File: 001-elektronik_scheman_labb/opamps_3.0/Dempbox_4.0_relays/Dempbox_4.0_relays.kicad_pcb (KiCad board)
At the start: 2 copper layers, 86 x 54.5 mm, 41 parts, among them J1 Test_probe, J10 Mätinstrument, J11 J_SW_SIGNAL, J2 TO_Focusrite_input, J3 OP_AMP_PWR, J4 Speaker, J9 Mätinstrument, U2 OPA134

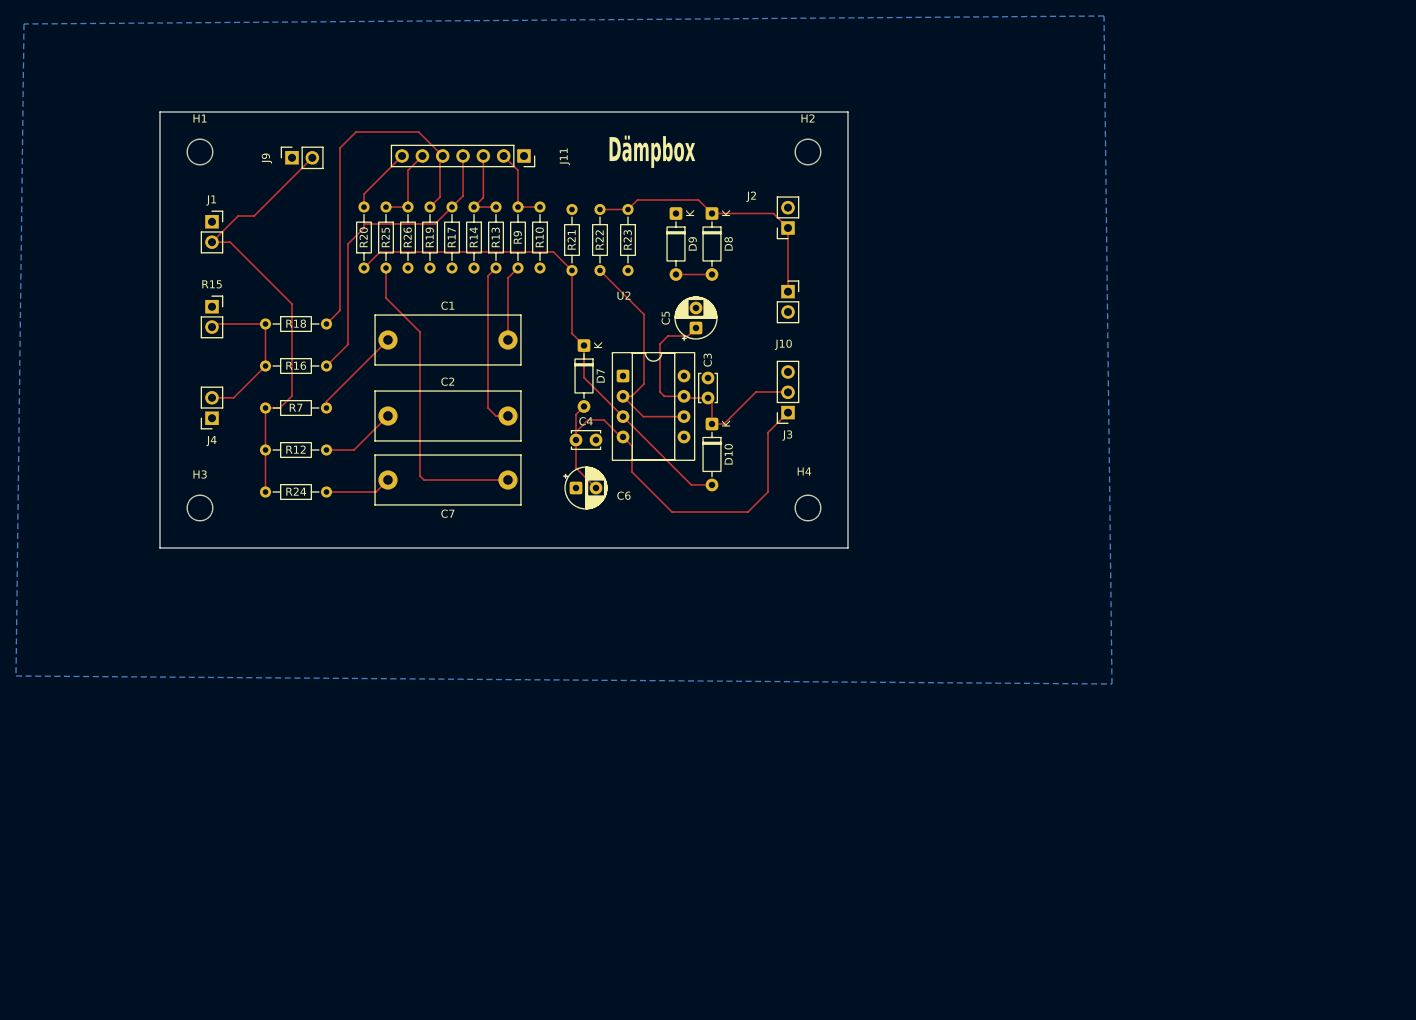
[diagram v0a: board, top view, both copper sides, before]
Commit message: Backup 2026-10-12
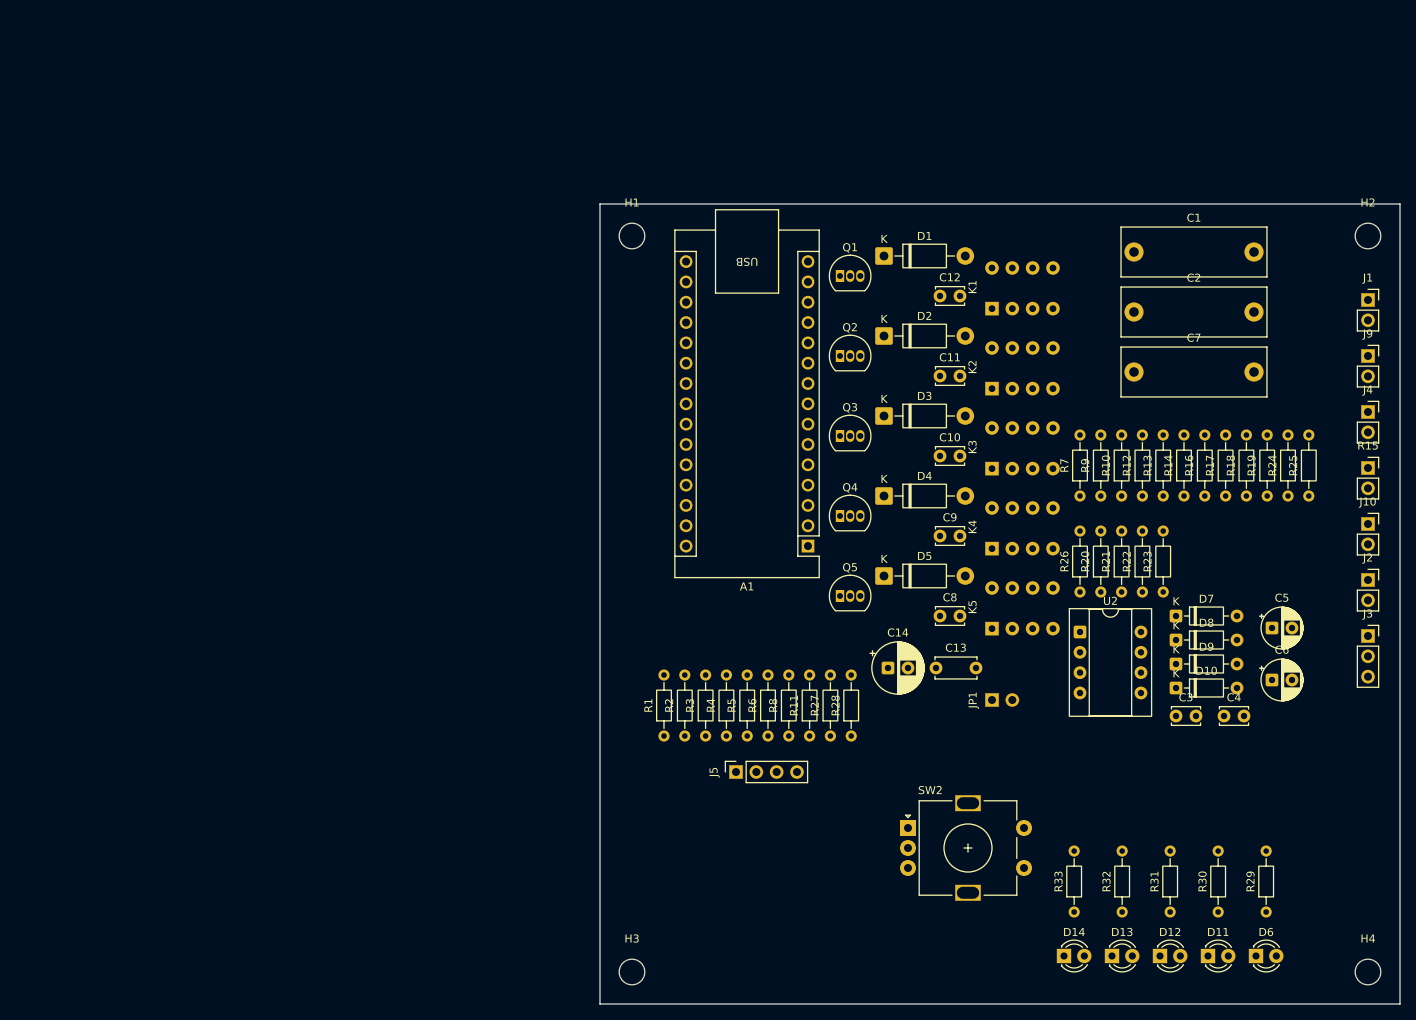
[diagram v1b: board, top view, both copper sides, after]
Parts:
- removed J11: J_SW_SIGNAL, Connector_PinSocket_2.54mm:PinSocket_1x07_P2.54mm_Vertical
- added A1: Arduino_Nano_esp32, Module:Arduino_Nano, F.Cu at (126.0, 92.8)
- added C10: 100nF, Capacitor_THT:C_Disc_D3.4mm_W2.1mm_P2.50mm, F.Cu at (142.5, 81.5)
- added C11: 100nF, Capacitor_THT:C_Disc_D3.4mm_W2.1mm_P2.50mm, F.Cu at (142.5, 71.5)
- added C12: 100nF, Capacitor_THT:C_Disc_D3.4mm_W2.1mm_P2.50mm, F.Cu at (142.5, 61.5)
- added C13: 10uF, Capacitor_THT:C_Disc_D5.0mm_W2.5mm_P5.00mm, F.Cu at (142.0, 108.0)
- added C14: 100uF, Capacitor_THT:CP_Radial_D6.3mm_P2.50mm, F.Cu at (136.0, 108.0)
- added C8: 100nF, Capacitor_THT:C_Disc_D3.4mm_W2.1mm_P2.50mm, F.Cu at (142.5, 101.5)
- added C9: 100nF, Capacitor_THT:C_Disc_D3.4mm_W2.1mm_P2.50mm, F.Cu at (142.5, 91.5)
- added D1: 1N4003, Diode_THT:D_DO-41_SOD81_P10.16mm_Horizontal, F.Cu at (135.5, 56.5)
- added D11: LED, LED_THT:LED_D3.0mm, F.Cu at (176.0, 144.0)
- added D12: LED, LED_THT:LED_D3.0mm, F.Cu at (170.0, 144.0)
- added D13: LED, LED_THT:LED_D3.0mm, F.Cu at (164.0, 144.0)
- added D14: LED, LED_THT:LED_D3.0mm, F.Cu at (158.0, 144.0)
- added D2: 1N4003, Diode_THT:D_DO-41_SOD81_P10.16mm_Horizontal, F.Cu at (135.5, 66.5)
- added D3: 1N4003, Diode_THT:D_DO-41_SOD81_P10.16mm_Horizontal, F.Cu at (135.5, 76.5)
- added D4: 1N4003, Diode_THT:D_DO-41_SOD81_P10.16mm_Horizontal, F.Cu at (135.5, 86.5)
- added D5: 1N4003, Diode_THT:D_DO-41_SOD81_P10.16mm_Horizontal, F.Cu at (135.5, 96.5)
- added D6: LED, LED_THT:LED_D3.0mm, F.Cu at (182.0, 144.0)
- added J5: OLCD_screen, Connector_PinSocket_2.54mm:PinSocket_1x04_P2.54mm_Vertical, F.Cu at (117.0, 121.0)
- added JP1: GND_LINK, Connector_PinHeader_2.54mm:PinHeader_1x02_P2.54mm_Vertical, F.Cu at (149.0, 112.0)
- added K1: G6K-2, Relay_THT:Relay_DPDT_Omron_G6K-2P, F.Cu at (149.0, 63.1)
- added K2: G6K-2, Relay_THT:Relay_DPDT_Omron_G6K-2P, F.Cu at (149.0, 73.1)
- added K3: G6K-2, Relay_THT:Relay_DPDT_Omron_G6K-2P, F.Cu at (149.0, 83.1)
- added K4: G6K-2, Relay_THT:Relay_DPDT_Omron_G6K-2P, F.Cu at (149.0, 93.1)
- added K5: G6K-2, Relay_THT:Relay_DPDT_Omron_G6K-2P, F.Cu at (149.0, 103.1)
- added Q1: 2N7000, Package_TO_SOT_THT:TO-92_Inline, F.Cu at (130.0, 59.0)
- added Q2: 2N7000, Package_TO_SOT_THT:TO-92_Inline, F.Cu at (130.0, 69.0)
- added Q3: 2N7000, Package_TO_SOT_THT:TO-92_Inline, F.Cu at (130.0, 79.0)
- added Q4: 2N7000, Package_TO_SOT_THT:TO-92_Inline, F.Cu at (130.0, 89.0)
- added Q5: 2N7000, Package_TO_SOT_THT:TO-92_Inline, F.Cu at (130.0, 99.0)
- added R1: 100, Resistor_THT:R_Axial_DIN0204_L3.6mm_D1.6mm_P7.62mm_Horizontal, F.Cu at (108.0, 116.5)
- added R11: 100K, Resistor_THT:R_Axial_DIN0204_L3.6mm_D1.6mm_P7.62mm_Horizontal, F.Cu at (126.2, 116.5)
- added R2: 100K, Resistor_THT:R_Axial_DIN0204_L3.6mm_D1.6mm_P7.62mm_Horizontal, F.Cu at (110.6, 116.5)
- added R27: 100, Resistor_THT:R_Axial_DIN0204_L3.6mm_D1.6mm_P7.62mm_Horizontal, F.Cu at (128.8, 116.5)
- added R28: 100K, Resistor_THT:R_Axial_DIN0204_L3.6mm_D1.6mm_P7.62mm_Horizontal, F.Cu at (131.4, 116.5)
- added R29: 220R, Resistor_THT:R_Axial_DIN0204_L3.6mm_D1.6mm_P7.62mm_Horizontal, F.Cu at (183.3, 138.5)
- added R3: 100, Resistor_THT:R_Axial_DIN0204_L3.6mm_D1.6mm_P7.62mm_Horizontal, F.Cu at (113.2, 116.5)
- added R30: 220R, Resistor_THT:R_Axial_DIN0204_L3.6mm_D1.6mm_P7.62mm_Horizontal, F.Cu at (177.3, 138.5)
- added R31: 220R, Resistor_THT:R_Axial_DIN0204_L3.6mm_D1.6mm_P7.62mm_Horizontal, F.Cu at (171.3, 138.5)
- added R32: 220R, Resistor_THT:R_Axial_DIN0204_L3.6mm_D1.6mm_P7.62mm_Horizontal, F.Cu at (165.3, 138.5)
- added R33: 220R, Resistor_THT:R_Axial_DIN0204_L3.6mm_D1.6mm_P7.62mm_Horizontal, F.Cu at (159.3, 138.5)
- added R4: 100K, Resistor_THT:R_Axial_DIN0204_L3.6mm_D1.6mm_P7.62mm_Horizontal, F.Cu at (115.8, 116.5)
- added R5: 100, Resistor_THT:R_Axial_DIN0204_L3.6mm_D1.6mm_P7.62mm_Horizontal, F.Cu at (118.4, 116.5)
- added R6: 100K, Resistor_THT:R_Axial_DIN0204_L3.6mm_D1.6mm_P7.62mm_Horizontal, F.Cu at (121.0, 116.5)
- added R8: 100, Resistor_THT:R_Axial_DIN0204_L3.6mm_D1.6mm_P7.62mm_Horizontal, F.Cu at (123.6, 116.5)
- added SW2: RotaryEncoder_Switch, Rotary_Encoder:RotaryEncoder_Alps_EC11E-Switch_Vertical_H20mm, F.Cu at (138.5, 128.0)
- moved R15 145.9 mm to (196.0, 83.0)
- moved J1 144.8 mm to (196.0, 62.0)
- moved J4 144.5 mm to (196.0, 76.0), turned to 0 degrees
- moved J9 136.8 mm to (196.0, 69.0), turned to 0 degrees
- moved R18 124.5 mm to (180.8, 86.5), turned to 90 degrees
- moved R25 120.9 mm to (188.6, 86.5), turned to 90 degrees
- moved R24 120.2 mm to (186.0, 86.5), turned to 90 degrees
- moved R16 118.5 mm to (175.6, 86.5), turned to 90 degrees
- moved R19 110.7 mm to (183.4, 86.5), turned to 90 degrees
- moved R12 109.8 mm to (167.8, 86.5), turned to 90 degrees
- moved R17 103.2 mm to (178.2, 86.5), turned to 90 degrees
- moved R7 102.4 mm to (160.0, 86.5), turned to 90 degrees
- moved R20 100.6 mm to (162.6, 98.5)
- moved R14 95.8 mm to (173.0, 86.5), turned to 90 degrees
- moved C2 94.2 mm to (166.8, 63.5)
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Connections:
- net /INT_1_100_OUT renamed INT_1_100_OUT
- net /INT_1_10_OUT renamed INT_1_10_OUT
- net /LOW_1_1_OUT renamed LOW_1_1_OUT
- net /SPK_1_100_OUT renamed SPK_1_100_OUT
- net /SPK_1_10_OUT renamed SPK_1_10_OUT
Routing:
- net Net-(D10-A): track 63.4 -> 0.00 mm
- net /INTPUT: track 56.0 -> 0.00 mm
- net /sound-card/12V-: track 55.9 -> 0.00 mm
- net SPK_1_10_OUT: track 44.8 -> 0.00 mm
- net Net-(C7-Pad1): track 39.0 -> 0.00 mm
- net SPK_1_100_OUT: track 38.5 -> 0.00 mm
- net /sound-card/audio_out: track 33.4 -> 0.00 mm
- net /sound-card/12V+: track 32.3 -> 0.00 mm
- net /sound-card/OP_AMP_OUT: track 28.4 -> 0.00 mm
- net Net-(C2-Pad2): track 20.8 -> 0.00 mm
- net /SPK_1_100: track 20.4 -> 0.00 mm
- net /INT_1_100: track 11.7 -> 0.00 mm
- net LOW_1_1_OUT: track 9.88 -> 0.00 mm
- net INT_1_100_OUT: track 9.87 -> 0.00 mm
- net INT_1_10_OUT: track 9.61 -> 0.00 mm
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- removed copper zone on B.Cu, net MEASURE_GND
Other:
- board size 86 x 54.5 mm -> 100 x 100 mm
- board text removed: "Dämpbox"
